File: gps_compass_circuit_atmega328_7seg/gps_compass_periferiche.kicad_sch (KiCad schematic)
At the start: 6 parts

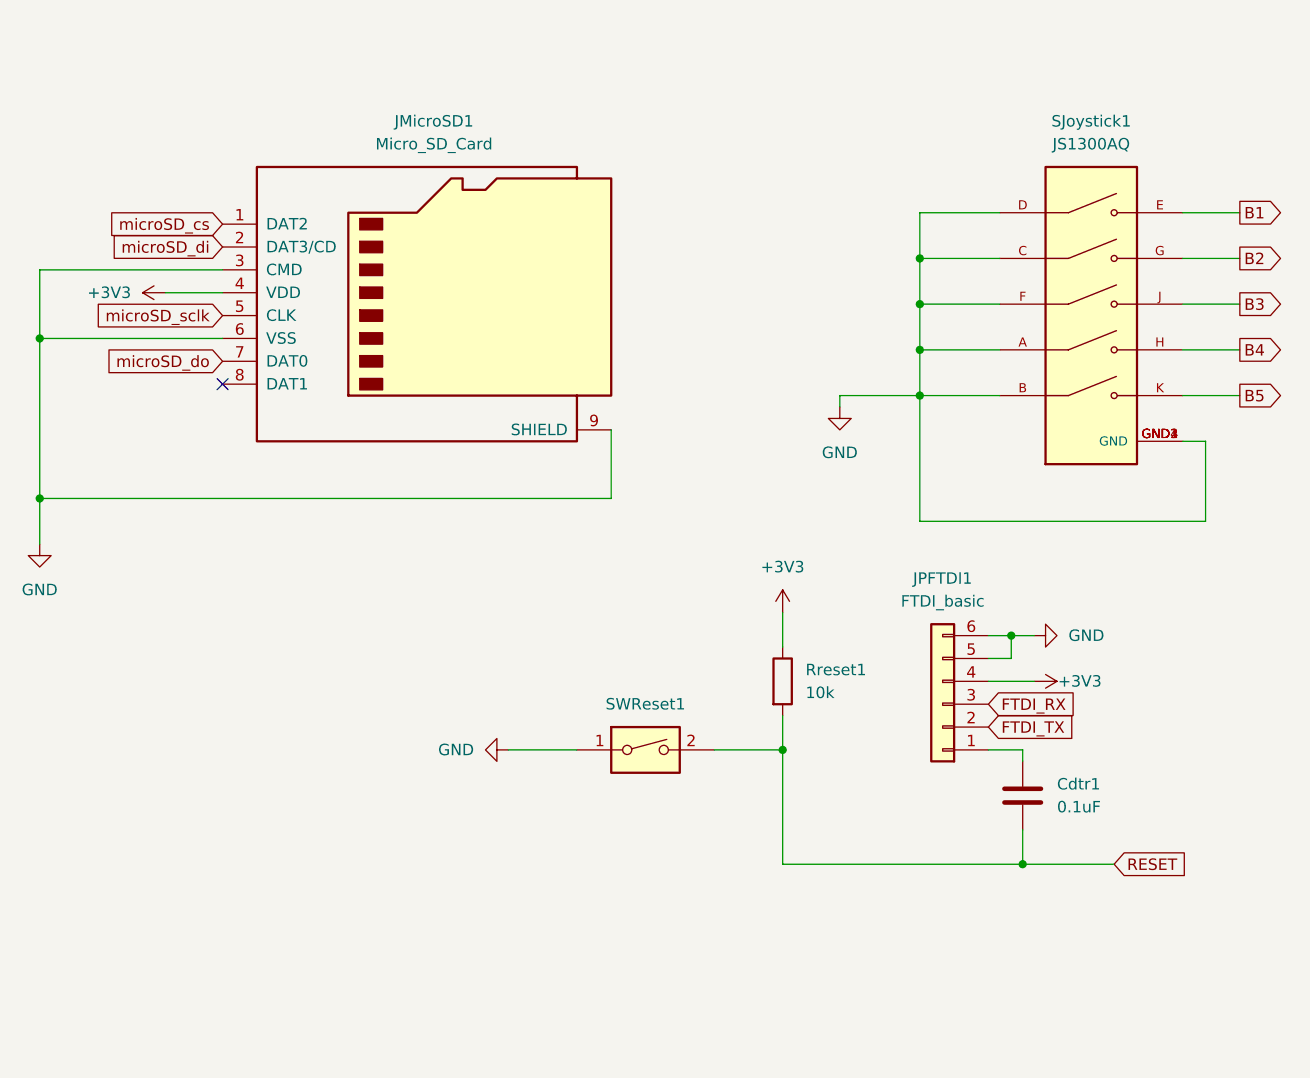
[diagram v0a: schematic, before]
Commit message: Aggiornato circuito
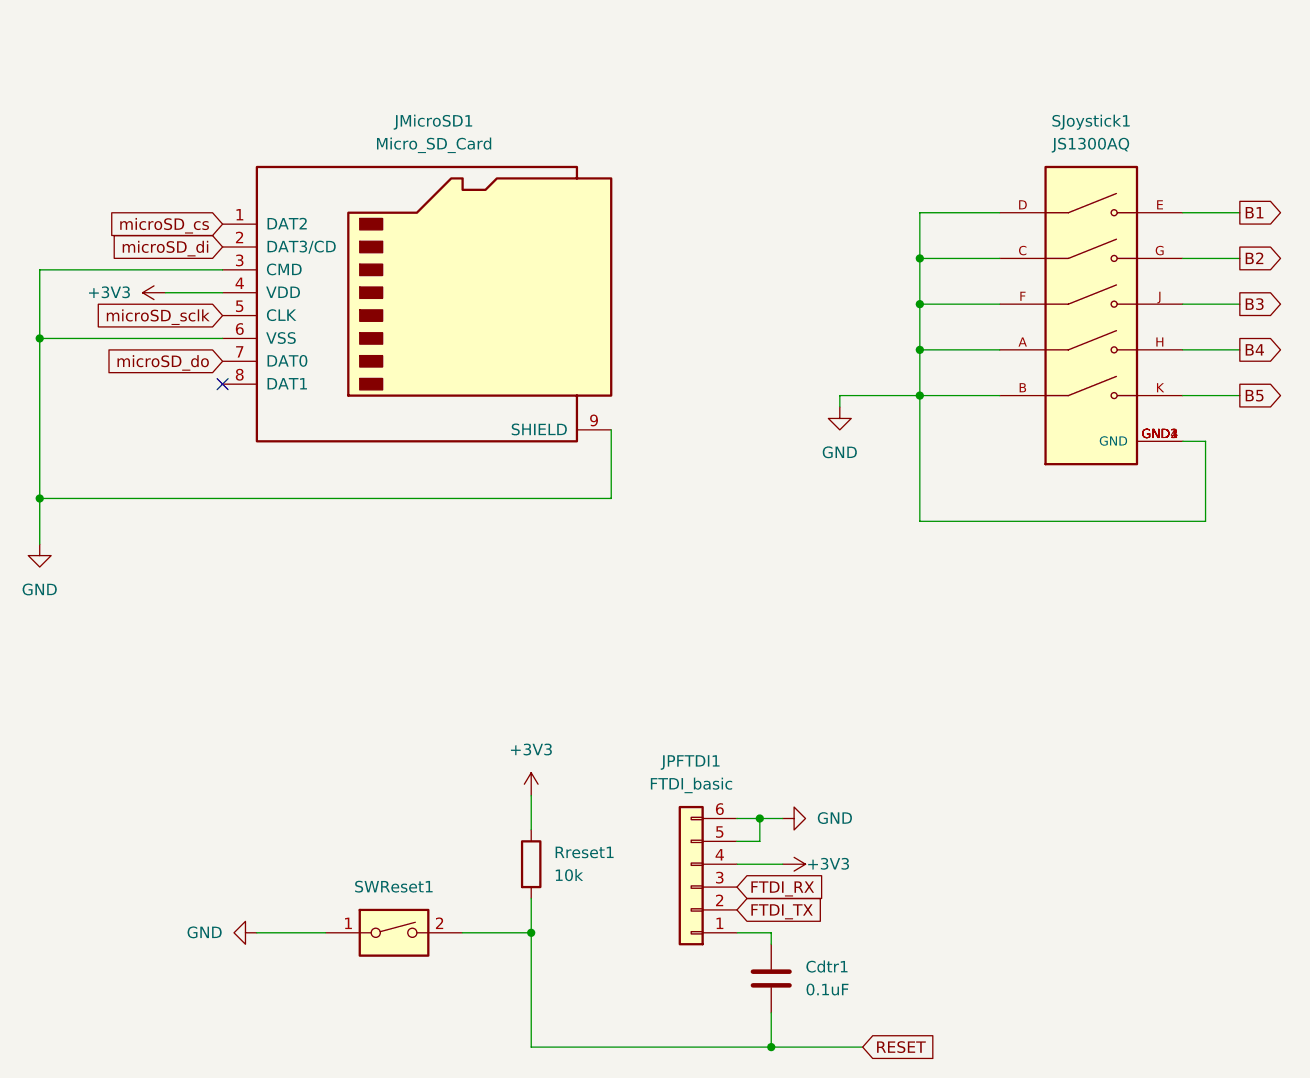
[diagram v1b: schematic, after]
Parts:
- SWReset1: footprint Button_Switch_SMD:SW_SPST_Omron_B3FS-101xP -> Button_Switch_THT:SW_PUSH_6mm
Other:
- moved on the sheet: Cdtr1, JPFTDI1, Rreset1, SWReset1

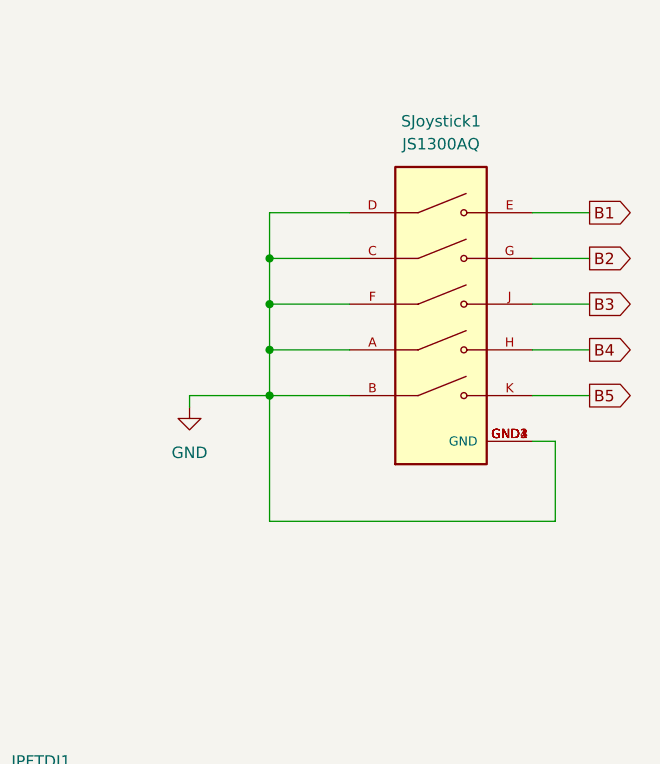
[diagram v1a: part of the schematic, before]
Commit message: Aggiornamenti vari
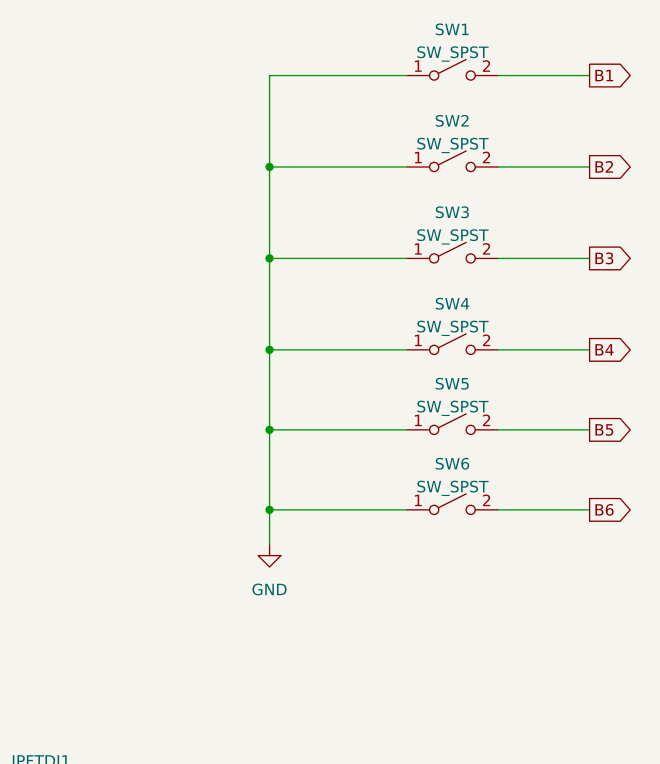
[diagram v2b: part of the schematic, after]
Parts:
- removed SJoystick1: JS1300AQ, SW_JS1300AQ, symbol JS1300AQ:JS1300AQ
- added SW1, SW2, SW3, SW4, SW5, SW6: SW_SPST, Button_Switch_THT:SW_PUSH_6mm, symbol Switch:SW_SPST
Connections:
- net B1: now also SW1.2 (B)
- net B2: now also SW2.2 (B)
- net B3: now also SW3.2 (B)
- net B4: now also SW4.2 (B)
- net B5: now also SW5.2 (B)
- net GND: now also SW1.1 (A), SW2.1 (A), SW3.1 (A), SW4.1 (A), SW5.1 (A), SW6.1 (A)
- new net B6: SW6.2 (B)
